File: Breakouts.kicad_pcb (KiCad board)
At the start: 2 copper layers, 189.9 x 66 mm, 13 parts, among them J1 Conn_01x08, J2 Conn_01x08, J3 Conn_01x08, J4 Conn_01x08, J5 Conn_02x04_Odd_Even, J6 Conn_01x06, J7 Conn_01x06, J8 AudioJack3, J9 Conn_01x03, K1 G5LE-1, U1 ESP-07, U2 AMS1117-3_3, U999999 ESP-12E

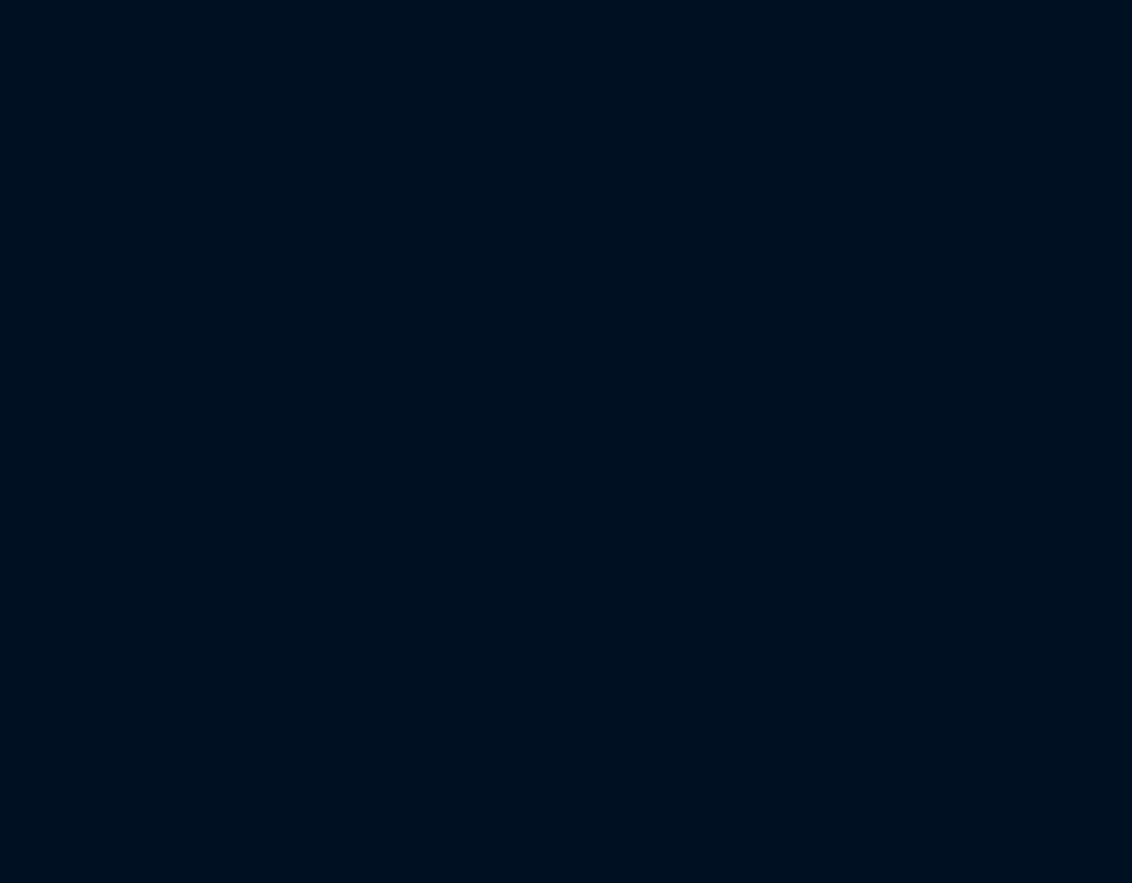
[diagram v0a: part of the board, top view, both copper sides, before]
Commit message: big audio jack
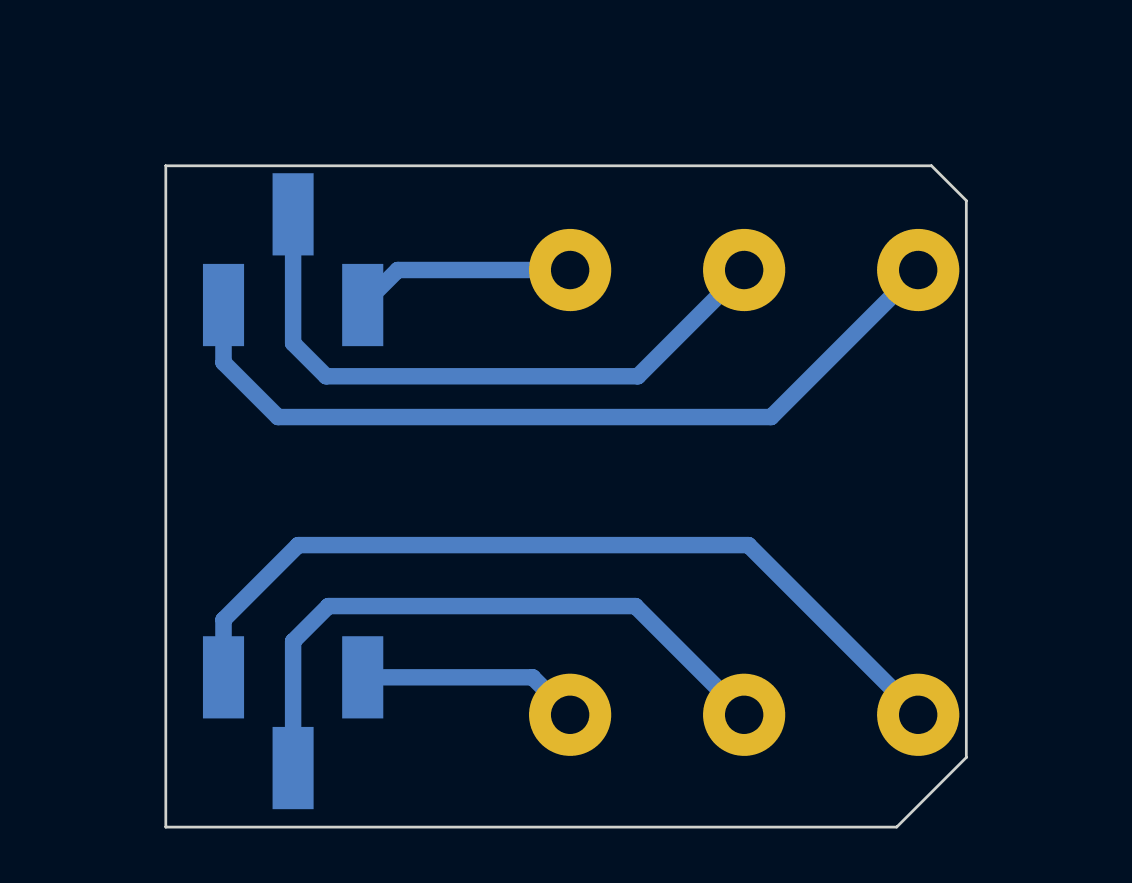
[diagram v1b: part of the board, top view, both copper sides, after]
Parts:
- added J10: AudioJack3_Switch, Connector_Audio:Jack_6.35mm_Neutrik_NMJ6HFD2_Horizontal, B.Cu at (209.1, 95.2)
- added J11: Conn_01x03, Connector_PinHeader_2.54mm:PinHeader_1x03_P2.54mm_Vertical_SMD_Pin1Left, B.Cu at (186.3, 94.9)
- added J12: Conn_01x03, Connector_PinHeader_2.54mm:PinHeader_1x03_P2.54mm_Vertical_SMD_Pin1Left, B.Cu at (186.3, 111.8)
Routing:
- net Net-(J12-Pin_1): track 0.00 -> 31.1 mm
- net Net-(J11-Pin_3): track 0.00 -> 30.5 mm
- net Net-(J11-Pin_2): track 0.00 -> 23.3 mm
- net Net-(J12-Pin_2): track 0.00 -> 23.3 mm
- net Net-(J12-Pin_3): track 0.00 -> 8.13 mm
- net Net-(J11-Pin_1): track 0.00 -> 8.10 mm
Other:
- board size 189.9 x 66 mm -> 189.9 x 96.5 mm
